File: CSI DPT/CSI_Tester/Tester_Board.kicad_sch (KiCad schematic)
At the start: 8 parts, among them Q1 UJ3N065025K3S, Q2 UJ3N065025K3S

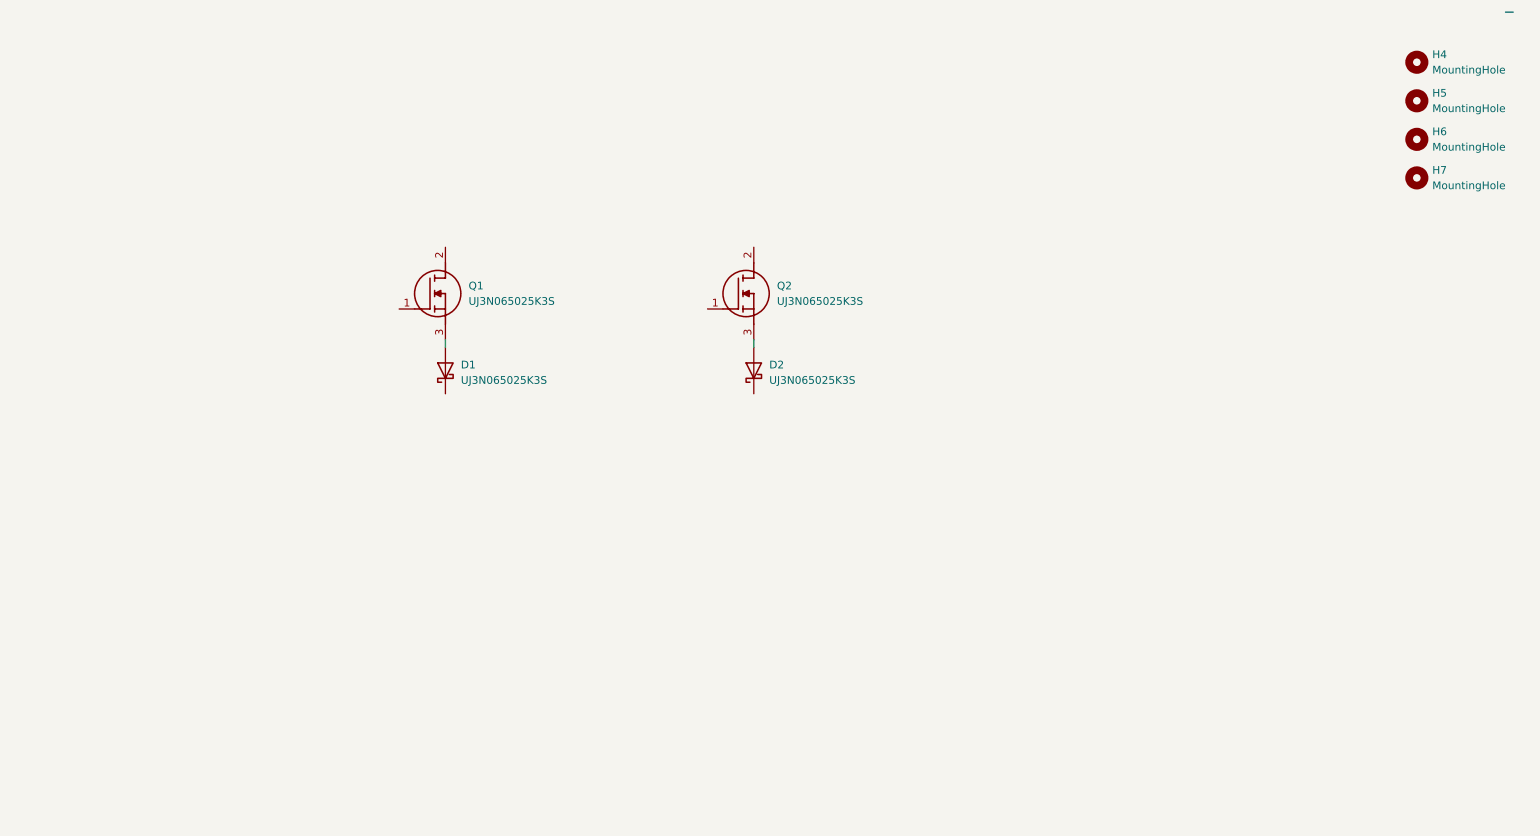
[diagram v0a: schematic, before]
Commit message: CSI Tester V1 Completed
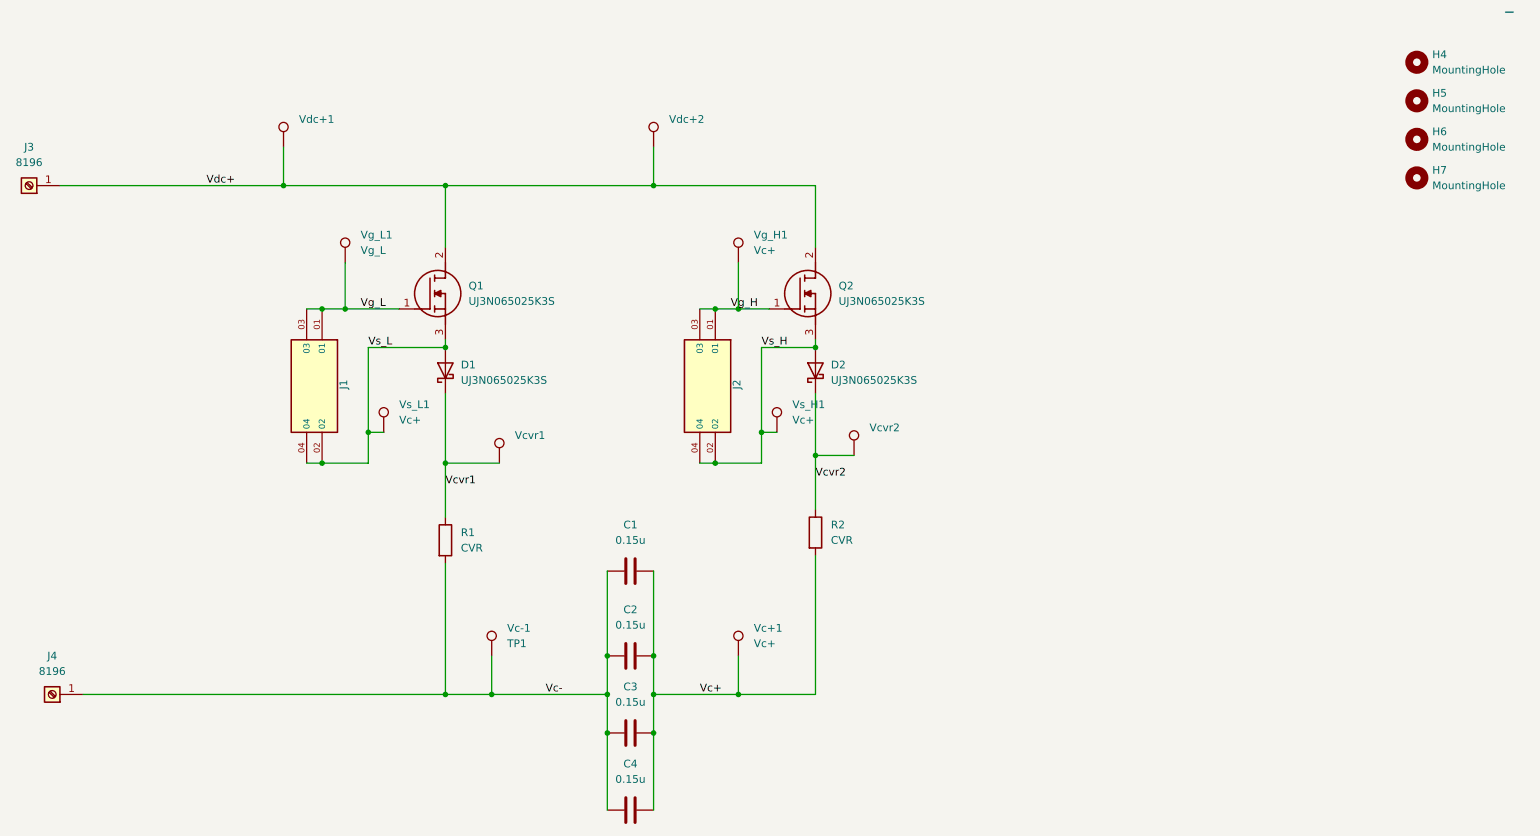
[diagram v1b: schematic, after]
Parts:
- added C1, C2, C3, C4: 0.15u, Capacitor_THT:C_Rect_L26.5mm_W10.5mm_P22.50mm_MKS4, symbol Device:C
- added J1, J2: TSM-102-01-SM-DV, VSI_DPT:SAMTEC_TSM-102-01-SM-DV, symbol VSI_DPT:TSM-102-01-SM-DV
- added J3, J4: 8196, CSI_DPT:CONN_8196_KEY, symbol VSI_DPT:8196
- added R1, R2: CVR, Resistor_THT:CVR_SSDN005, symbol Device:R
- added Vc+1, Vg_H1, Vs_H1, Vs_L1: Vc+, TestPoint:TestPoint_Pad_D2.0mm, symbol Connector:TestPoint
- added Vc-1: TP1, TestPoint:TestPoint_Pad_D2.0mm, symbol Connector:TestPoint
- added Vcvr1, Vcvr2, Vdc+1, Vdc+2: ~, TestPoint:TestPoint_Pad_D2.0mm, symbol Connector:TestPoint
- added Vg_L1: Vg_L, TestPoint:TestPoint_Pad_D2.0mm, symbol Connector:TestPoint
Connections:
- net Vg_H: now reaches Q2.1 (G)
- net Vg_H: now also J2.01, J2.03, Vg_H1.1
- net Vdc+: now reaches Q2.2 (D)
- net Vdc+: now also Q1.2 (D), J3.1, Vdc+1.1, Vdc+2.1
- net Vs_H: now reaches D2.2 (A), Q2.3 (S)
- net Vs_H: now also J2.02, J2.04, Vs_H1.1
- net Vcvr2: now reaches D2.1 (K)
- net Vcvr2: now also R2.1, Vcvr2.1
- net Vcvr1: now reaches D1.1 (K)
- net Vcvr1: now also R1.1, Vcvr1.1
- net Vs_L: now reaches D1.2 (A), Q1.3 (S)
- net Vs_L: now also J1.02, J1.04, Vs_L1.1
- net Vg_L: now reaches Q1.1 (G)
- net Vg_L: now also J1.01, J1.03, Vg_L1.1
- new net Vc+: C1.2, C2.2, C3.2, C4.2, R2.2, Vc+1.1
- new net Vc-: C1.1, C2.1, C3.1, C4.1, J4.1, R1.2, Vc-1.1
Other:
- moved on the sheet: D2, Q2
